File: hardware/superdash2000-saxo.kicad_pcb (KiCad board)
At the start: 2 copper layers, 76.2 x 55.9 mm, 21 parts, among them IC1 MAX4617CPE+, J1 Molex 34691-0161, U1 L7805, U2 TLV2372

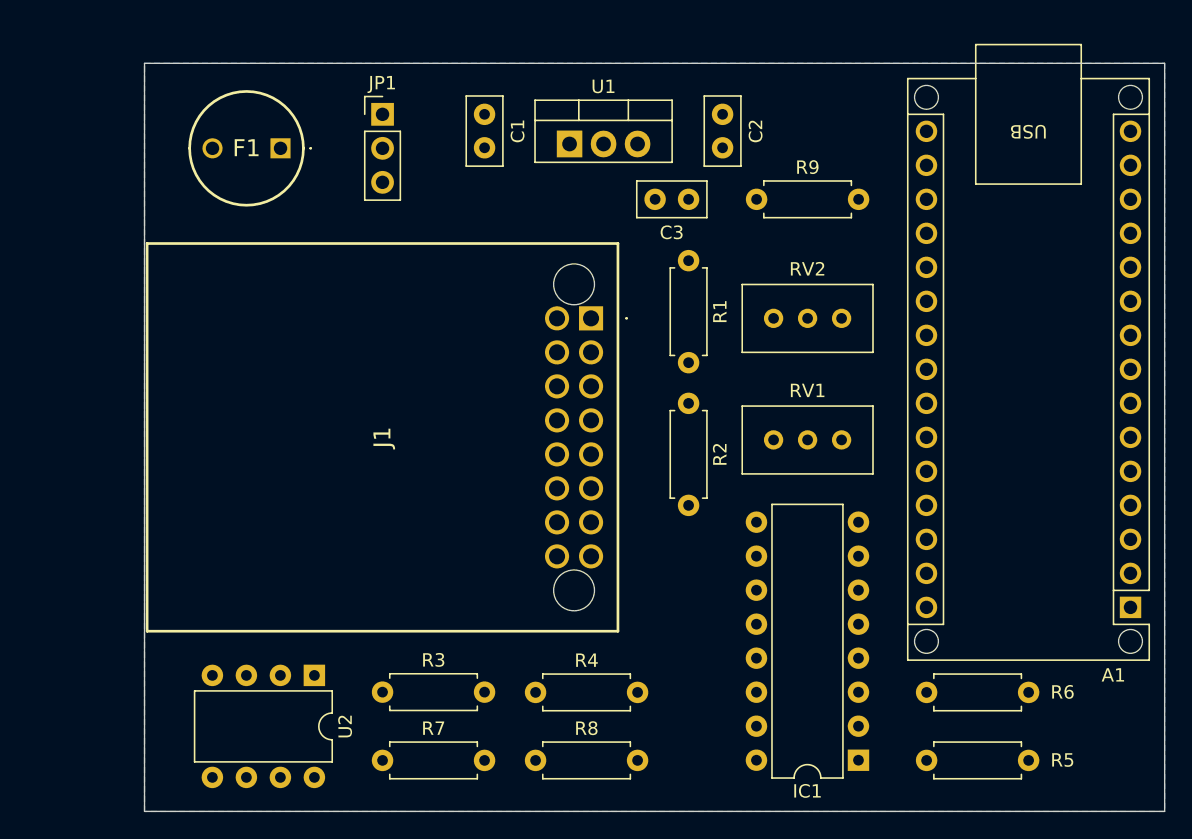
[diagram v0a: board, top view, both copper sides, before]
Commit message: hardware: Update pcb
Signed-off-by: Thomas Antonini <antonini.thomas@gmail.com>
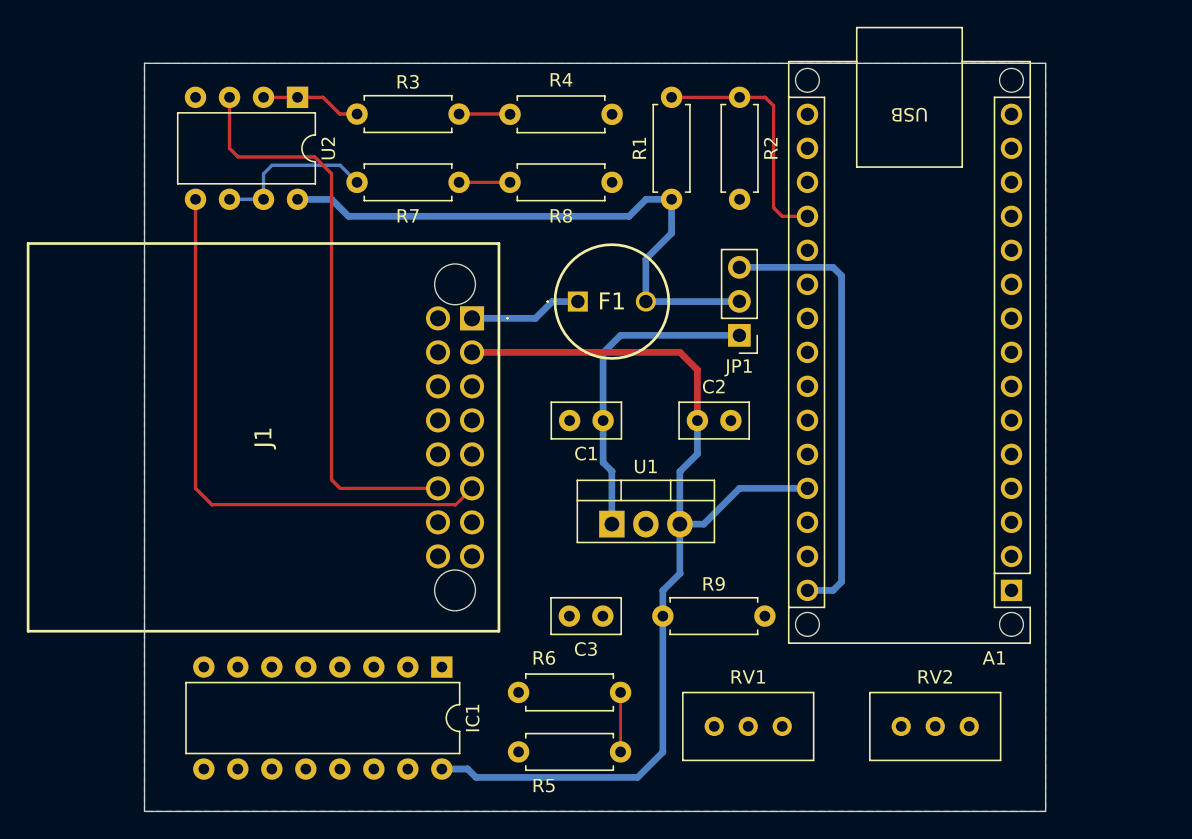
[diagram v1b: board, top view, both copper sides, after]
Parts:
- moved R4 43.6 mm to (64.1, 58.4), turned to 180 degrees
- moved R7 43.2 mm to (45.1, 63.5)
- moved R8 43.2 mm to (56.5, 63.5)
- moved R3 43.2 mm to (45.1, 58.4)
- moved U2 43.2 mm to (40.6, 57.1)
- moved RV2 31.9 mm to (90.8, 104.1)
- moved R9 31.9 mm to (67.9, 95.9)
- moved IC1 31.9 mm to (51.4, 99.7), turned to -90 degrees
- moved C3 31.8 mm to (63.4, 95.9)
- moved JP1 31.4 mm to (73.6, 74.9), turned to 180 degrees
- moved R5 30.5 mm to (57.1, 106.0)
- moved R6 30.5 mm to (57.1, 101.6)
- moved U1 28.6 mm to (64.1, 89.0)
- moved F1 25.0 mm to (61.6, 72.4), turned to 0 degrees
- moved C1 24.5 mm to (63.5, 81.3), turned to 180 degrees
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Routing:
- net +5V: track 0.00 -> 75.2 mm
- net VCC: track 0.00 -> 43.8 mm
- net /WATER_TEMP: track 0.00 -> 43.3 mm
- net /DIMMER: track 0.00 -> 43.3 mm
- net /VIN: track 0.00 -> 33.6 mm
- net Net-(C1-Pad1): track 0.00 -> 23.8 mm
- net /A0: track 0.00 -> 18.3 mm
- net Net-(R7-Pad1): track 0.00 -> 12.2 mm
- net +BATT: track 0.00 -> 8.44 mm
- net Net-(R3-Pad1): track 0.00 -> 7.50 mm
- net /LCD_BRIGHTNESS+: track 0.00 -> 4.45 mm
- net /D3: track 0.00 -> 3.82 mm
- net /D4: track 0.00 -> 3.81 mm
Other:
- board size 76.2 x 55.9 mm -> 67.3 x 55.9 mm
